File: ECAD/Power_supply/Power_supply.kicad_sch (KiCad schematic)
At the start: 40 parts, among them J1 Barrel_Jack_Switch, J2 Conn_01x06, Q1 DMP3037LSS-13, SW1 SW_Push_DPDT, U1 LM317_TO-220, U2 LM317_TO-220

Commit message: Progressed PCB layout.
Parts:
- J2: footprint Connector_PinHeader_2.54mm:PinHeader_1x06_P2.54mm_Horizontal -> Connector_PinSocket_2.54mm:PinSocket_1x06_P2.54mm_Vertical; Status OK -> (none)
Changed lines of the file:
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@@
 			)
 		)
-		(property "Footprint" "Connector_PinHeader_2.54mm:PinHeader_1x06_P2.54mm_Horizontal"
+		(property "Footprint" "Connector_PinSocket_2.54mm:PinSocket_1x06_P2.54mm_Vertical"
 			(at 189.23 111.76 0)
 			(effects
@@
 			)
 		)
-		(property "Status" "OK"
+		(property "Status" ""
 			(at 189.23 111.76 0)
 			(effects

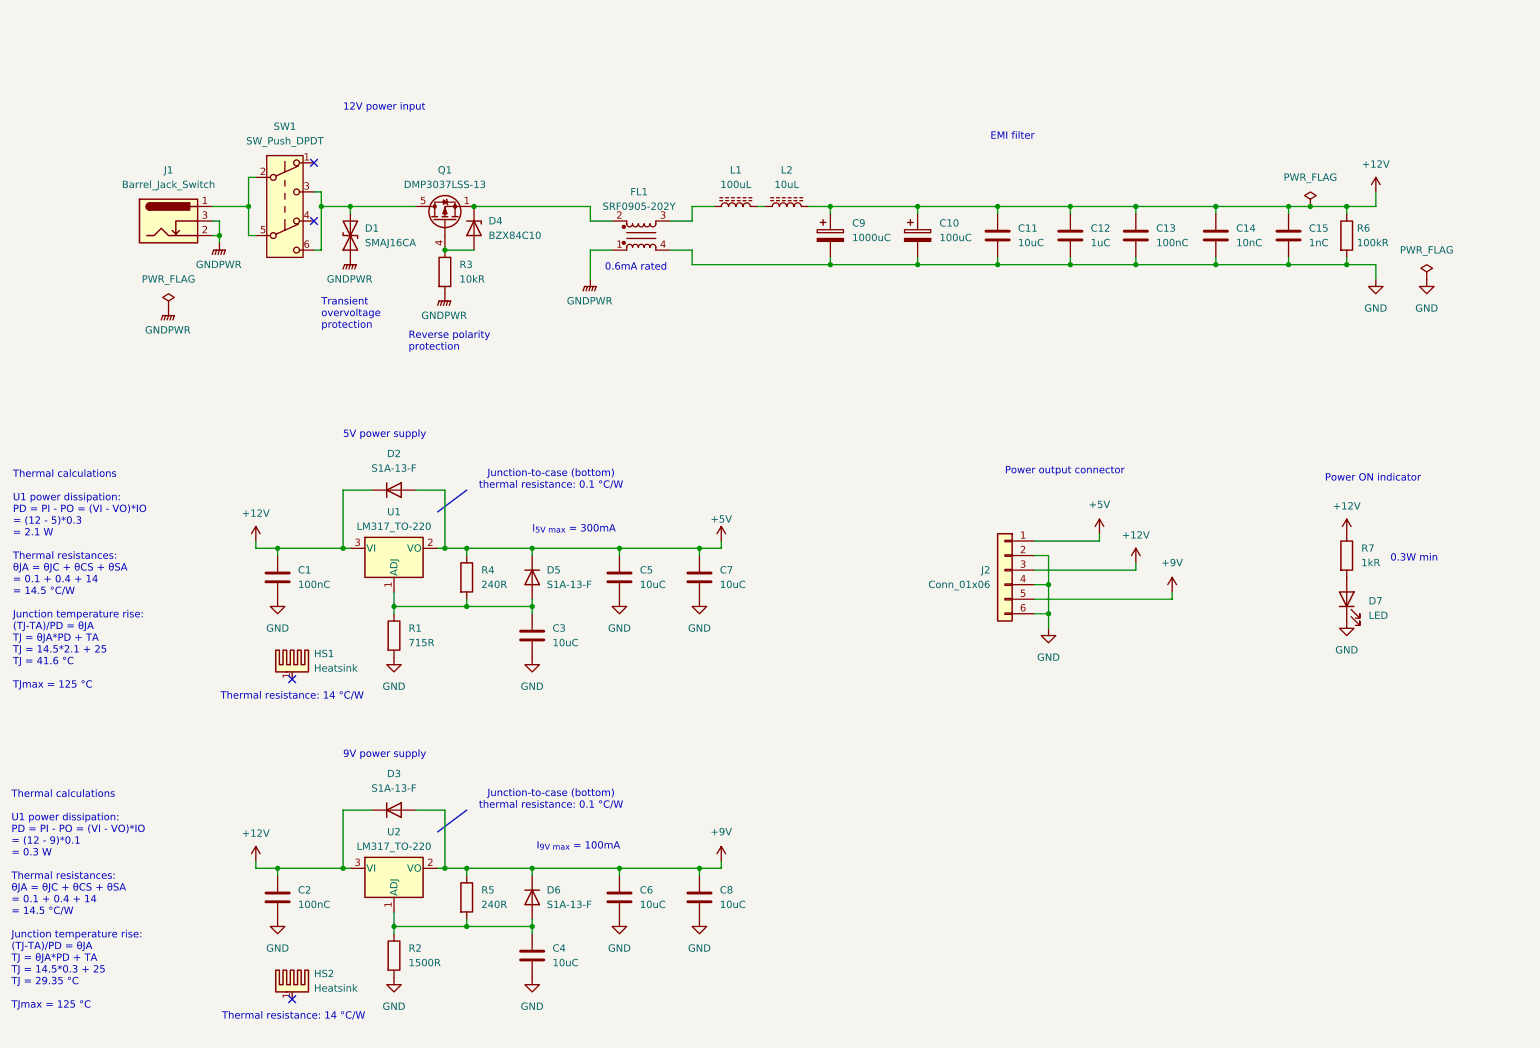
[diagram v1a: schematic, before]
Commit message: Updated the schematic.
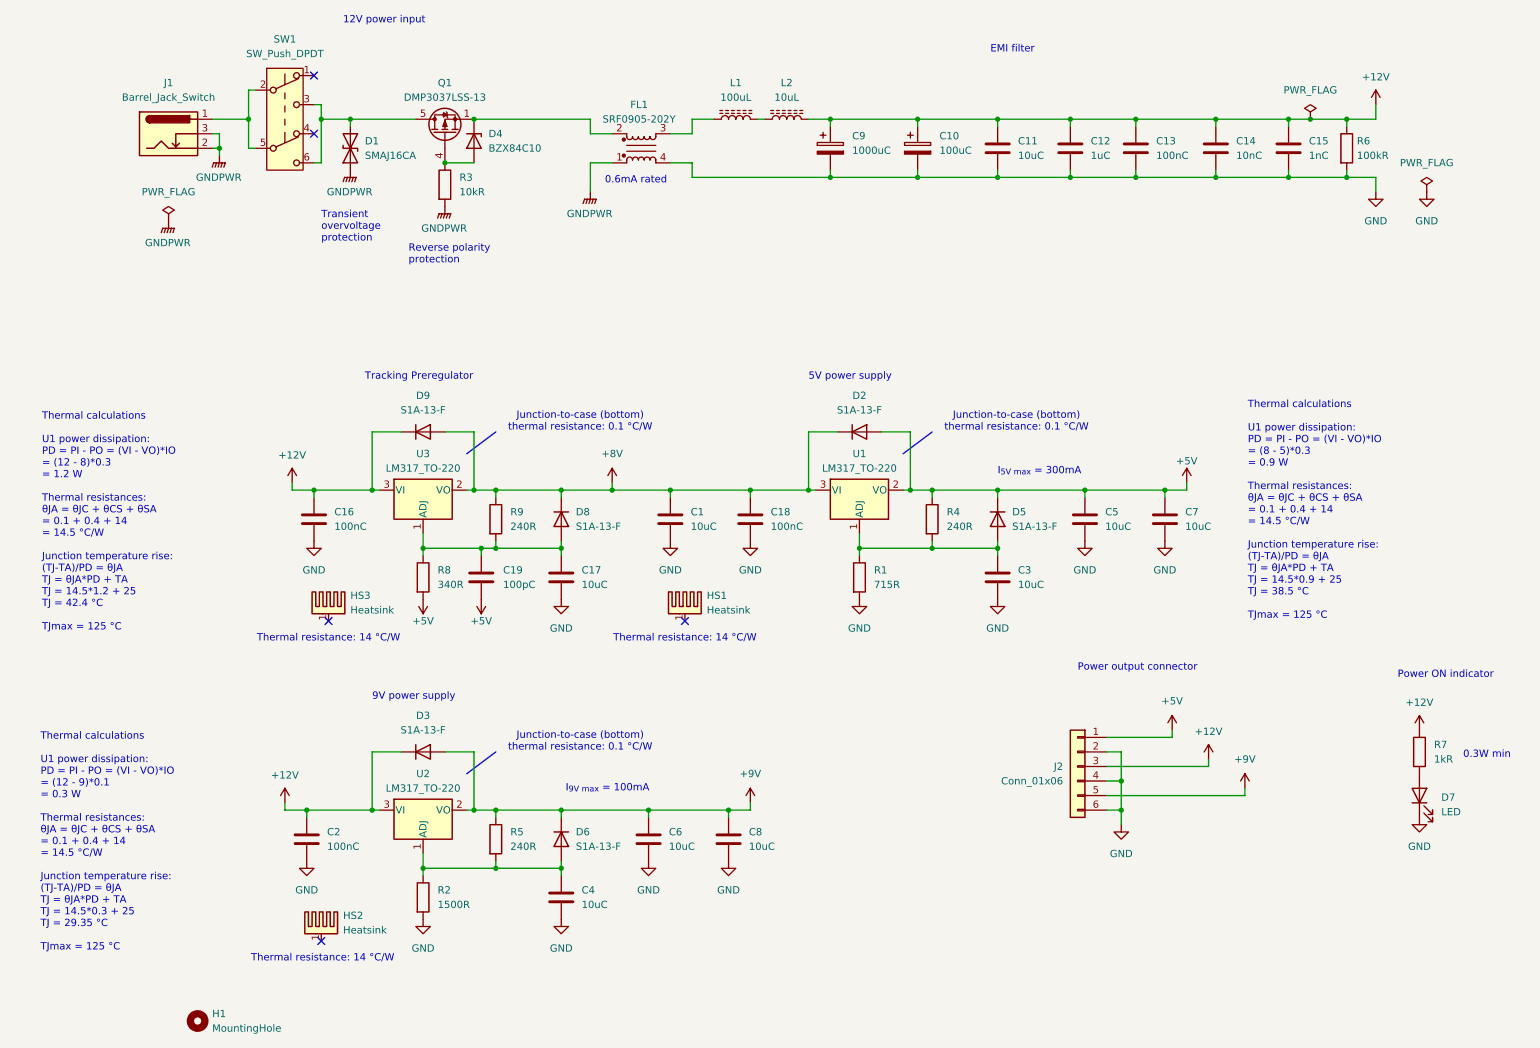
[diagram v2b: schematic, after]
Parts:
- added C16, C18: 100nC, Capacitor_SMD:C_1206_3216Metric, symbol Device:C
- added C17: 10uC, Capacitor_SMD:C_1206_3216Metric, symbol Device:C
- added C19: 100pC, Capacitor_SMD:C_0805_2012Metric, symbol Device:C
- added D8, D9: S1A-13-F, Diode_SMD:D_SMA, symbol Diode:SM4001
- added H1: MountingHole, symbol Mechanical:MountingHole
- added HS3: Heatsink, Heatsink:Heatsink_Fischer_SK104-STC-STIC_35x13mm_2xDrill2.5mm, symbol Mechanical:Heatsink_Pad
- added R8: 340R, Resistor_SMD:R_0805_2012Metric, symbol Device:R
- added R9: 240R, Resistor_SMD:R_0805_2012Metric, symbol Device:R
- added U3: LM317_TO-220, Package_TO_SOT_THT:TO-220-3_Vertical, symbol Regulator_Linear:LM317_TO-220
- C1: value 100nC -> 10uC; MPN CC1206KRX7R9BB104 -> CL31A106KBHNNNE
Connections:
- net +12V: now also C16.1, D9.1 (K), U3.3 (VI); no longer C1.1, D2.1 (K), U1.3 (VI)
- net +5V: now also C19.2, R8.2
- net GND: now also C16.2, C17.2, C18.2
- new net: C17.1, C19.1, D8.2 (A), R8.1, R9.2, U3.1 (ADJ)
- new net +8V: C1.1, C18.1, D2.1 (K), D8.1 (K), D9.2 (A), R9.1, U1.3 (VI), U3.2 (VO)
- no-connect marks 4 -> 5
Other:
- note added: "Thermal calculations U1 power dissipation: PD = PI - PO = (VI - VO)*IO = (12 - 8)*0.3 = 1.2 W Thermal resistances: θJA = θJC + θCS + θSA = 0.1 + 0.4 + 14 = 14.5 °C/W Junction temperature rise: (TJ-TA)/PD = θJA TJ = θJA*PD + TA TJ = 14.5*1.2 + 25 TJ = 42.4 °C TJmax = 125 °C"
- note added: "Thermal calculations U1 power dissipation: PD = PI - PO = (VI - VO)*IO = (8 - 5)*0.3 = 0.9 W Thermal resistances: θJA = θJC + θCS + θSA = 0.1 + 0.4 + 14 = 14.5 °C/W Junction temperature rise: (TJ-TA)/PD = θJA TJ = θJA*PD + TA TJ = 14.5*0.9 + 25 TJ = 38.5 °C TJmax = 125 °C"
- note added: "Tracking Preregulator"
- note removed: "Thermal calculations U1 power dissipation: PD = PI - PO = (VI - VO)*IO = (12 - 5)*0.3 = 2.1 W Thermal resistances: θJA = θJC + θCS + θSA = 0.1 + 0.4 + 14 = 14.5 °C/W Junction temperature rise: (TJ-TA)/PD = θJA TJ = θJA*PD + TA TJ = 14.5*2.1 + 25 TJ = 41.6 °C TJmax = 125 °C"
- moved on the sheet: C10, C11, C12, C13, C14, C15, C2, C3, C4, C5, C6, C7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
